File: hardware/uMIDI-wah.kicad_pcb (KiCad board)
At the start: 2 copper layers, 55 x 30 mm, 39 parts, among them Q1 BSS138, U1 uA741CDR, X1 9V, X2 uMIDI, X3 Input, X4 Output

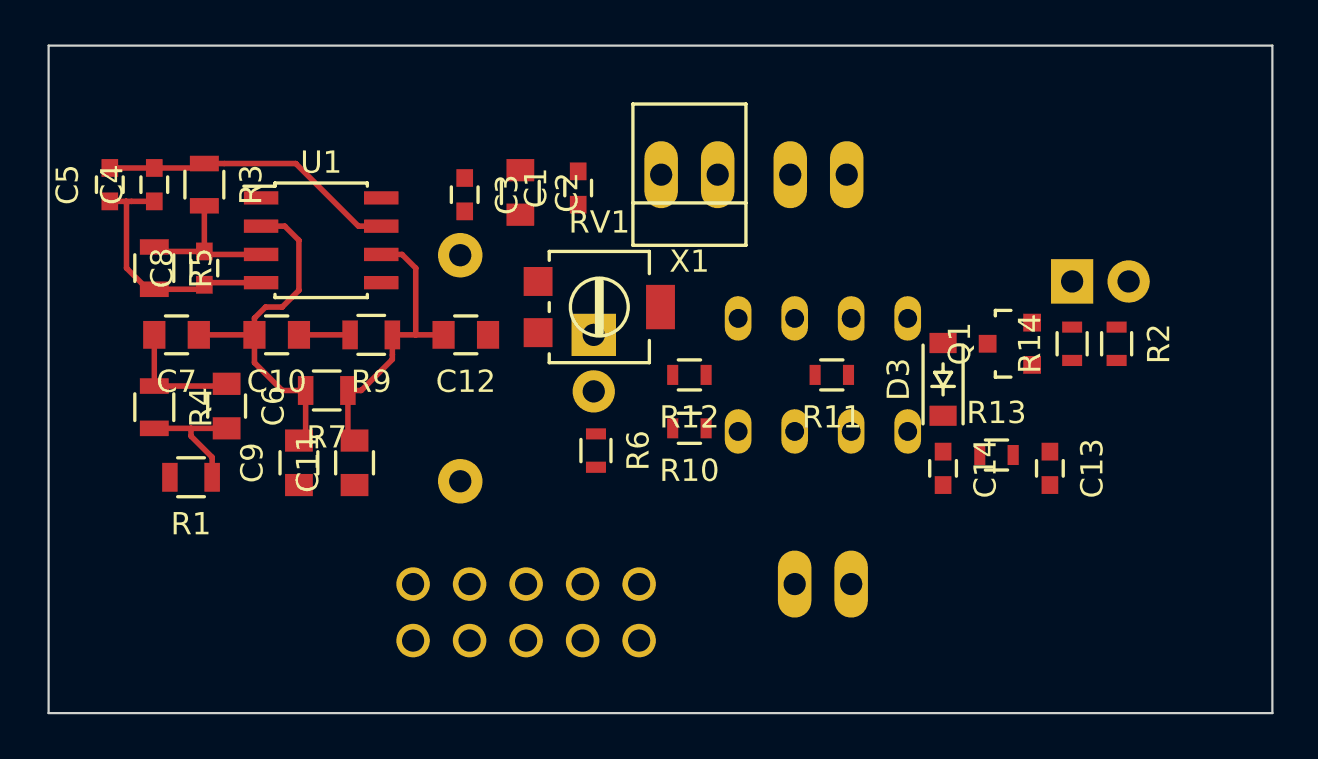
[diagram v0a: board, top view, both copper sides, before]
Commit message: Place and route
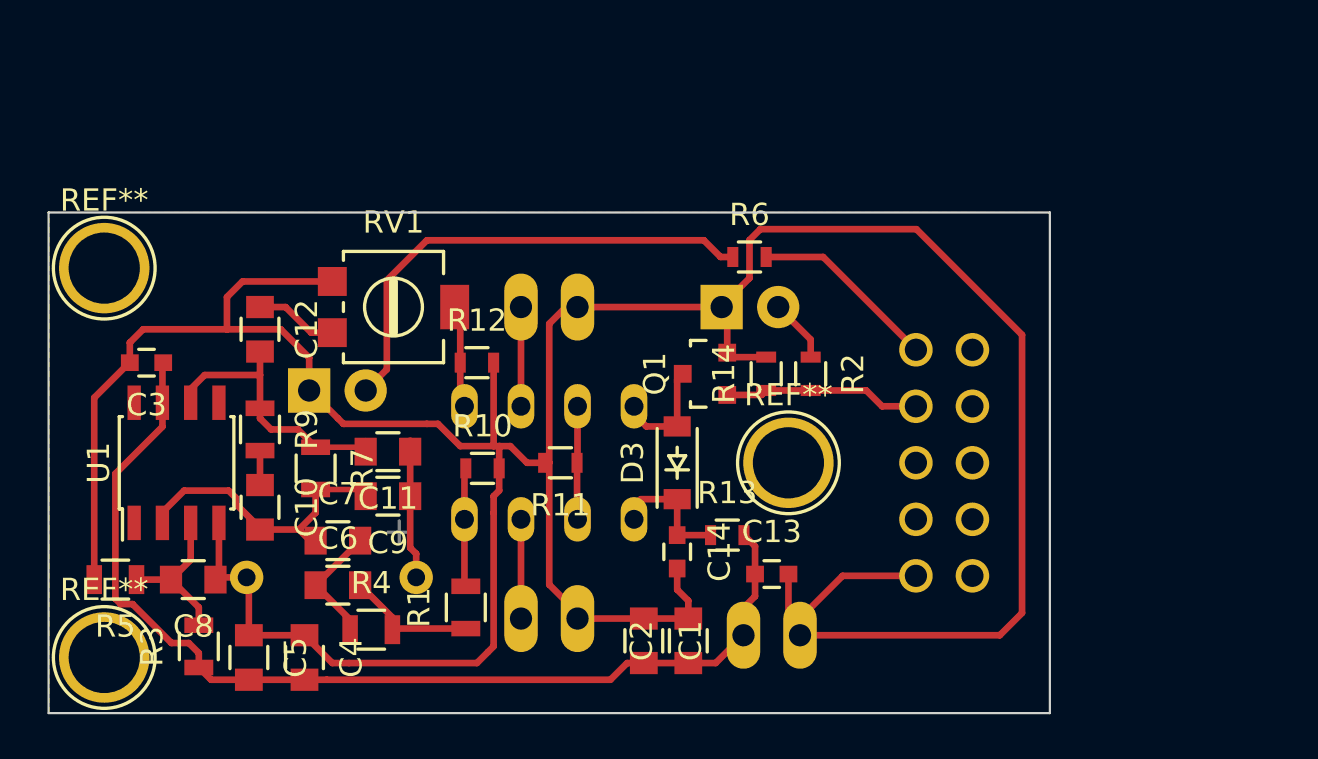
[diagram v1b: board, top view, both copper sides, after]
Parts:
- added REF**: 1pin, Connect:1pin, F.Cu at (213.2, 138.8)
- added REF**: 1pin, Connect:1pin, F.Cu at (182.5, 147.5)
- added REF**: 1pin, Connect:1pin, F.Cu at (182.5, 130.0)
- C1, C4, C5, C8: footprint Capacitors_SMD:C_0603 -> Capacitors_SMD:C_0805
- R8: value Photores -> LDR 05; footprint Resistors_ThroughHole:Resistor_Horizontal_RM10mm -> Capacitors_Elko_ThroughHole:Elko_vert_20x10mm_RM7.5
- X1: moved to B.Cu
- moved C4 22.3 mm to (191.5, 147.5), turned to 270 degrees
- moved C5 22.2 mm to (189.0, 147.5), turned to 270 degrees
- moved C2 21.5 mm to (208.8, 146.8), turned to 90 degrees
- moved X1 21.0 mm to (212.5, 146.5)
- moved R3 20.8 mm to (186.8, 147.0), turned to 90 degrees
- moved C1 20.6 mm to (206.8, 146.8), turned to 270 degrees
- moved X2 20.0 mm to (220.2, 138.8), turned to 270 degrees
- moved C3 16.2 mm to (184.4, 134.2), turned to 180 degrees
- moved D1 15.8 mm to (210.2, 131.8)
- moved R5 14.1 mm to (183.0, 144.0), turned to 180 degrees
- moved C8 14.0 mm to (186.5, 144.0), turned to 180 degrees
- moved R4 14.0 mm to (194.5, 146.2), turned to 0 degrees
- moved R14 13.8 mm to (212.2, 134.8)
- moved R2 13.8 mm to (214.2, 134.8)
- moved Q1 13.8 mm to (209.5, 134.8)
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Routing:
- net GND: track 11.6 -> 156.4 mm
- net (no net): track 109.5 -> 0.00 mm
- net +9V: track 13.4 -> 47.5 mm
- net Net-(D2-Pad2): track 0.00 -> 21.9 mm
- net /True bypass/Ctrl: track 0.00 -> 8.86 mm
- net /PWM: track 0.00 -> 8.46 mm
- net Net-(C11-Pad1): track 0.00 -> 6.26 mm
- net /True bypass/relais_p: track 0.00 -> 5.78 mm
- net /True bypass/FX_Send: track 0.00 -> 5.43 mm
- net /True bypass/FX_Return: track 0.00 -> 5.35 mm
- net /True bypass/bypass: track 0.00 -> 5.10 mm
- net /True bypass/relais_n: track 0.00 -> 4.99 mm
- net /True bypass/Loop_Out: track 0.00 -> 4.46 mm
- net /True bypass/Loop_In: track 0.00 -> 4.46 mm
- net Net-(C12-Pad1): track 0.00 -> 3.73 mm
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- added copper zone on F.Cu, net GND
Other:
- board size 55 x 30 mm -> 45 x 22.5 mm
